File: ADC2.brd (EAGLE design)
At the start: 90 x 99 mm, 192 parts, among them CON1 USB-A, CON2 SWD_CON, IC1 STM32G431, IC10 NJM11100, IC11 TAR5SB33, IC12 LM4562, IC13 LM4562, IC14 NJM12888F18, IC15 AZ1117-3.3, IC16 -9V, IC17 +9V, IC18 LM4562, IC19 TC7WH74FU, IC2 7404, IC20 NJM2845-33, IC21 -5V, IC3 ESP32-WROVER, IC4 LME49721, IC5 TL431, IC6 AD4001, IC7 OCT_BUFFER-SO6, IC8 OCT_BUFFER-SO6, IC9 TAR5SB33, J2 SJ-1608, J4 SJ-1608, J5 SJ-2012, J6 IN1_DC, J7 SJ-1608, J8 short, J9 SJ-2012, SW1 Gain, X1 12MHz

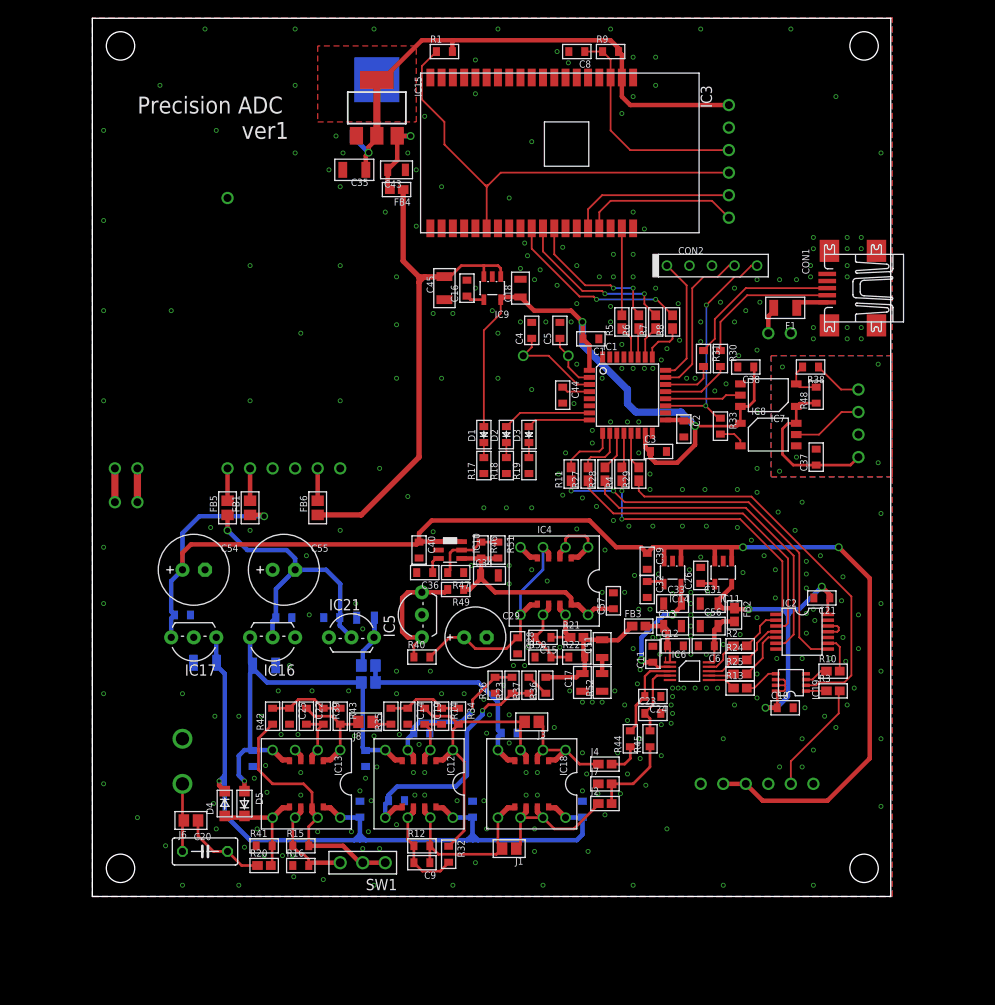
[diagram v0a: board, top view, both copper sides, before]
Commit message: ver2修正
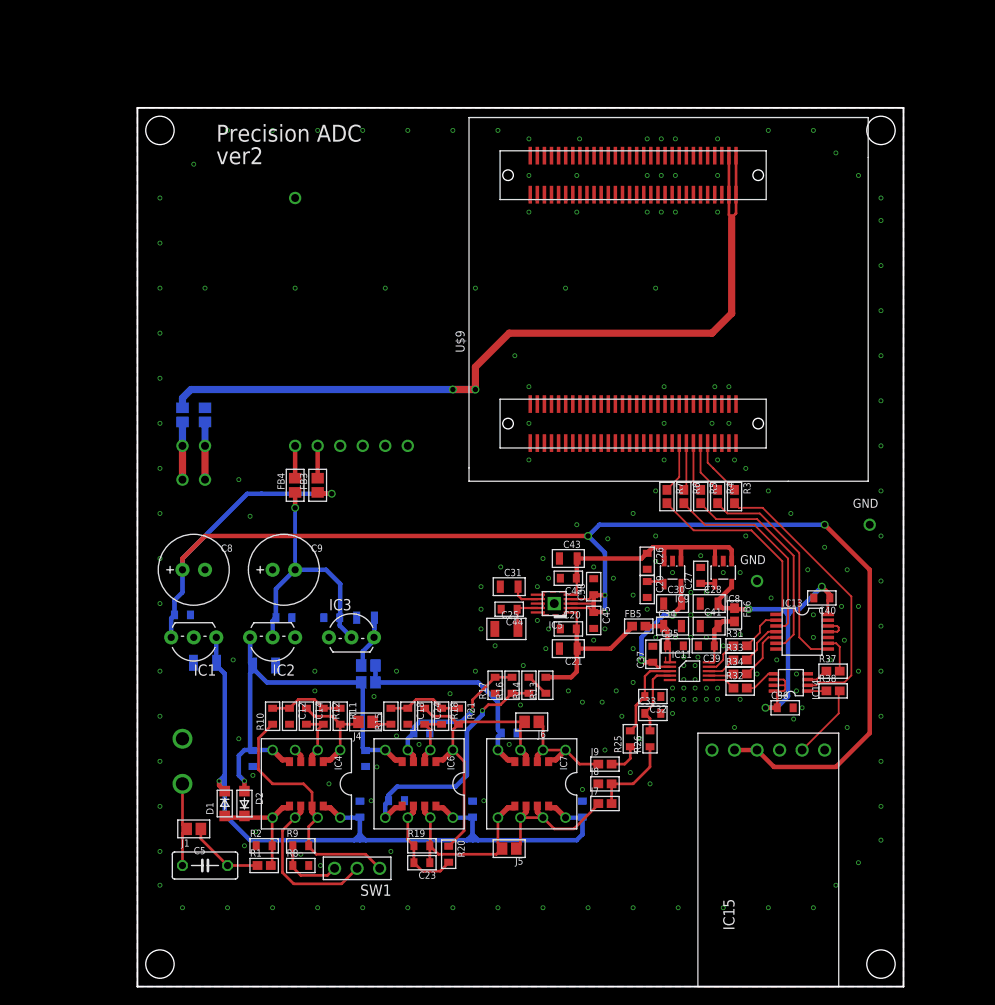
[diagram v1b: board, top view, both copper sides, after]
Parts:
- removed C46, C47: 10u, my_rcl:3216
- removed C48, C49, C50, C52, C53, C57, C59: 0.1u, my_rcl:1608
- removed C51, R52: DNP, my_rcl:2012
- removed C54, C55: 100u, my_rcl:E2,5-8
- removed C56, C58: 10u, my_rcl:2012
- removed CON1: USB-A, my_connector:UX60A-MB-5ST
- removed CON2: SWD_CON, my_connector:SWD_CON
- removed D3: ERR, my_rcl:D1608
- removed D4, D5: CLAMP, my_rcl:SOD123
- removed F1: 0.5A, my_rcl:3216
- removed IC10: NJM11100, my_ic:SOT23-6
- removed IC12, IC18: LM4562, my_ic:DIL8-SOP8
- removed IC16: -9V, my_ic:TO-92
- removed IC17: +9V, my_ic:TO-92
- removed IC19: TC7WH74FU, my_ic:SSOP8-P-0.65
- removed IC20: NJM2845-33, my_ic:P-HSIP3_2.30A
- removed IC21: -5V, my_ic:TO-92
- removed R22, R23, R35, R36, R39, R42, R43, R48, R49, R50: 1k, my_rcl:1608
- removed R24, R27, R28, R29: 37, my_rcl:1608-J
- removed R30, R44, R45: 22, my_rcl:1608
- removed R40, R46, R51: 10k, my_rcl:1608
- removed R41: 100k, my_rcl:1608
- removed R47: 1.5k, my_rcl:1608
- removed TP10: ESP_EN, my_connector:TESTPIN
- removed TP11: ESP_BOOT, my_connector:TESTPIN
- removed TP12: ESP_TX, my_connector:TESTPIN
- removed TP13, TP20, TP27, TP28, TP29: GND, my_connector:TESTPIN
- removed TP14: ESP_RX, my_connector:TESTPIN
- removed TP24: VDD_OSC, my_connector:TESTPIN
- removed TP25: OSC_EN, my_connector:TESTPIN
- removed TP26: OSC_OUT, my_connector:TESTPIN
- removed TP6: UART_RX, my_connector:TESTPIN
- removed TP7: UART_GND, my_connector:TESTPIN
- removed TP8: UART_TX, my_connector:TESTPIN
- removed TP9: +3V3D, my_connector:TESTPIN
- removed X1: 12MHz, my_rcl:HC49/S
- added U$9: FPGA_CORE_BOARD, my_ic:FPGA_CORE_BOARD
- C12: value 3300p -> 470p
- C13: value 10u -> 0.1u; device my_rcl:2012 -> my_rcl:1608
- C14, C24: value 470p -> 100p
- C15: value DNP -> 10u; device my_rcl:1608 -> my_rcl:2012
- C16: value 0.1u -> 10u; device my_rcl:1608 -> my_rcl:3216
- C17: device my_rcl:2012 -> my_rcl:3216
- C18, C33: value 10u -> 470p; device my_rcl:2012 -> my_rcl:1608
- C19, C22: value 100p -> 0.1u
- C20: value 10u -> 1u; device my_rcl:C050 -> my_rcl:1608
- C21, C30, C41: value 0.1u -> 10u; device my_rcl:1608 -> my_rcl:2012
- C23: value 470p -> DNP
- C25: value 470p -> 10u; device my_rcl:1608 -> my_rcl:3216
- C28: value 1u -> 10u; device my_rcl:1608 -> my_rcl:2012
- C29: value 100u -> 0.1u; device my_rcl:E2.5-6.5 -> my_rcl:1608
- C3: value 0.01u -> 0.1u
- C32: value 0.1u -> 470p
- C35: value 10u -> 3300p; device my_rcl:3216 -> my_rcl:1608
- C38, C42: value 0.1u -> 1u
- C4: value 22p -> 0.1u
- C44: value 0.1u -> DNP
- C45: value 10u -> 1u; device my_rcl:3216 -> my_rcl:1608
- C5: value 22p -> 10u; device my_rcl:1608 -> my_rcl:C050
- C8: value 0.1u -> 100u; device my_rcl:1608 -> my_rcl:E2,5-8
- C9: value DNP -> 100u; device my_rcl:1608 -> my_rcl:E2,5-8
- D1: value PWR -> CLAMP; device my_rcl:D1608 -> my_rcl:SOD123
- D2: value OK -> CLAMP; device my_rcl:D1608 -> my_rcl:SOD123
- FB2, FB3, FB4: value FB -> FB-2012; device my_rcl:1608-J -> my_rcl:2012-J
- FB5, FB6: value FB-2012 -> FB; device my_rcl:2012-J -> my_rcl:1608-J
- IC1: value STM32G431 -> +9V; device my_ic:TQFP32-08 -> my_ic:TO-92
- IC11: value TAR5SB33 -> AD4001; device my_ic:SOT23-5 -> my_ic:MSOP10
- IC13: value LM4562 -> 7404; device my_ic:DIL8-SOP8 -> my_ic:TSSOP14
- IC14: value NJM12888F18 -> TC7WH74FU; device my_ic:SOT23-5 -> my_ic:SSOP8-P-0.65
- IC15: value AZ1117-3.3 -> OSC; device my_ic:SOT223 -> my_ic:MY_OSC
- IC2: value 7404 -> -9V; device my_ic:TSSOP14 -> my_ic:TO-92
- IC3: value ESP32-WROVER -> -5V; device my_ic:ESP32-WROVER -> my_ic:TO-92
- IC4: value LME49721 -> LM4562
- IC5: value TL431 -> AK1110; device my_ic:TO-92 -> my_ic:PLP10
- IC6: value AD4001 -> LM4562; device my_ic:MSOP10 -> my_ic:DIL8-SOP8
- IC7: value OCT_BUFFER-SO6 -> LM4562; device my_ic:SO6 -> my_ic:DIL8-SOP8
- IC8: value OCT_BUFFER-SO6 -> TAR5SB33; device my_ic:SO6 -> my_ic:SOT23-5
- IC9: value TAR5SB33 -> NJM12888F18
- J1: value (none) -> IN1_DC
- J2: value SJ-1608 -> SJ-2012; device my_rcl:1608-J -> my_rcl:2012-J
- J3: value (none) -> SJ-2012
- J4: value SJ-1608 -> short; device my_rcl:1608-J -> my_rcl:2012-J
- J6: value IN1_DC -> SJ-2012
- J8: value short -> SJ-1608; device my_rcl:2012-J -> my_rcl:1608-J
- J9: value SJ-2012 -> SJ-1608; device my_rcl:2012-J -> my_rcl:1608-J
- R1: value 10k -> 10; device my_rcl:1608 -> my_rcl:1608-J
- R10, R11, R13, R8: value 37 -> 1k; device my_rcl:1608-J -> my_rcl:1608
- R15: value 10k -> 1k
- R17, R18, R19: value 1.5k -> 1k
- R2: value 37 -> 100k; device my_rcl:1608-J -> my_rcl:1608
- R20: value 10 -> 1k; device my_rcl:1608-J -> my_rcl:1608
- R21: value short -> 1k; device my_rcl:1608-J -> my_rcl:1608
- R25: value 37 -> 22; device my_rcl:1608-J -> my_rcl:1608
- R26: value 1k -> 22
- R3, R4, R5, R6, R7: value 37 -> 22
- R31: value 22 -> 37; device my_rcl:1608 -> my_rcl:1608-J
- R32, R33, R34, R37, R38: value 1k -> 37; device my_rcl:1608 -> my_rcl:1608-J
- TP4: value VBUS -> GND
- TP5: value UART_3V3 -> GND
- moved R9 96.1 mm to (23.5, 5.71)
- moved R1 94.0 mm to (19.4, 3.49)
- moved IC15 84.8 mm to (76.2, 16.5), turned to 90 degrees
- moved R8 74.2 mm to (23.5, 3.49), turned to 0 degrees
- moved C8 72.6 mm to (11.4, 36.8), turned to 0 degrees
- moved C5 72.4 mm to (12.7, 3.49), turned to 0 degrees
- moved C10 68.7 mm to (10.2, 31.8), flipped to the bottom, turned to 180 degrees
- moved C35 64.7 mm to (65.7, 28.3), turned to 0 degrees
- moved FB2 63.8 mm to (12.7, 54.3), flipped to the bottom
- moved R10 63.4 mm to (20.3, 20.3), turned to 90 degrees
- moved C2 61.2 mm to (18.1, 15.6), flipped to the bottom, turned to 90 degrees
- moved IC2 59.7 mm to (20.3, 29.2), turned to 180 degrees
- moved C1 59.1 mm to (30.2, 9.84), flipped to the bottom, turned to 90 degrees
- moved IC13 58.5 mm to (80.0, 29.8), turned to 270 degrees
- moved IC3 58.3 mm to (29.2, 29.2), turned to 0 degrees
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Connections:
- removed net +3V3: C1.2, C18.1, C2.1, C3.1, C38.1, D1.A, IC1.1, IC1.15, IC1.17, IC7.6, IC8.1, IC9.5
- removed net +3V3D: C35.1, IC15.2, IC15.4, IC20.3, IC3.2, R1.2, R9.2, TP9.1
- removed net +5.3V: C34.1, C57.1, IC10.4, IC4.1-8, IC4.2-8, R46.2, R49.1, R51.2
- removed net +5VD: C45.1, FB4.1, FB6.2, IC9.1, IC9.3
- removed net ADC1+: J4.2, R44.1
- removed net ADC1-: J2.2, J7.2, R45.1
- removed net ESP_BOOT: IC3.25, R1.1, TP11.1
- removed net ESP_EN: C8.1, IC3.3, R9.1, TP10.1
- removed net ESP_RX: IC3.34, TP14.1
- removed net ESP_TX: IC3.35, TP12.1
- removed net N$23: C15.1, IC4.1-7, IC4.2-7, R21.1
- removed net N$27: D1.K, R17.2
- removed net N$32: CON1.2, R30.1
- removed net N$33: CON1.3, R31.1
- removed net N$34: IC8.3, R33.2
- removed net N$35: IC7.3, R38.2, R48.2
- removed net N$36: IC1.10, R27.2
- removed net N$37: IC1.11, R28.2
- removed net N$39: IC13.1-6, IC13.2-6, R15.1, R16.2, SW1.3
- removed net N$40: D2.K, R18.2
- removed net N$46: D3.K, R19.2
- removed net N$50: D3.A, IC1.8
- removed net N$51: C16.1, IC9.4
- removed net N$52: C24.2, IC6.3, R44.2
- removed net N$53: C23.1, IC6.4, R45.2
- removed net N$54: D2.A, IC1.7
- removed net N$58: C15.2, IC4.1-6, IC4.2-6, R22.1, R50.2
- removed net N$60: IC5.1, IC5.3, R40.1, R49.2
- removed net N$61: C36.1, IC10.3
- removed net N$62: IC10.5, R46.1, R47.2, R51.1
- removed net N$63: C28.1, C29.+, IC4.1-3, IC4.1-5, IC4.2-3, IC4.2-5, R40.2
- removed net N$64: IC4.1-1, IC4.1-2, IC4.2-1, IC4.2-2
- removed net N$65: F1.2, TP4.1
- removed net N$66: C44.1, IC1.4
- removed net N$69: C43.1, FB4.2, IC15.3, IC20.1
- removed net N$72: FB6.1, TP1.1
- removed net N$73: C51.2, R52.2
- removed net SPI_CS: IC3.29, R8.2
- removed net SPI_MISO: IC3.31, R6.2
- removed net SPI_MOSI: IC3.37, R5.2
- removed net SPI_SCK: IC3.30, R7.2
- removed net STM_RX: IC1.20, IC7.5
- removed net STM_TX: CON2.5, IC1.19, R33.1
- removed net SWCLK: CON2.1, IC1.24
- removed net SWDIO: CON2.4, IC1.23
- removed net UART_3V3: C37.1, IC7.1, IC8.6, R48.1, TP5.1
- removed net UART_GND: C37.2, IC8.4, TP7.1
- removed net UART_RX: R38.1, TP6.1
- removed net UART_TX: IC8.5, TP8.1
- removed net USB_DM: IC1.21, R30.2
- removed net USB_DP: IC1.22, R31.2
- removed net VBUS: CON1.1, F1.1
- new net +5V: C26.1, C42.1, C43.1, IC5.5, IC8.1, IC8.3, IC9.1, IC9.3
- new net ADC+: J9.2, R25.1
- new net ADC+_LPF: C32.2, IC11.3, R25.2
- new net ADC-: J7.2, J8.2, R26.1
- new net ADC-_LPF: C33.1, IC11.4, R26.2
- new net VIN: FB1.1, U$9.117, U$9.118, U$9.119, U$9.120
- net +1V8: now also C30.1, C37.1, IC11.2, IC9.5; no longer C11.1, C33.1, IC14.5, IC6.2
- net +3V3A: now also C28.1, C36.1, C40.1, FB6.1, IC13.14, IC14.6, IC14.7, IC14.8, IC8.5; no longer C10.1, C21.1, C31.1, FB2.1, IC11.5, IC19.6, IC19.7, IC19.8, IC2.14
- net +9V: now also C1.1, C16.1, C3.1, C6.1, D1.2, IC1.1, IC4.1-8, IC4.2-8, IC6.1-8, IC6.2-8, IC7.1-8, IC7.2-8; no longer C41.1, C46.1, C48.1, C7.1, D4.2, IC12.1-8, IC12.2-8, IC13.1-8, IC13.2-8, IC17.1, IC18.1-8, IC18.2-8
- net -5V: now also C15.2, IC3.3, J3.1; no longer C58.2, IC21.3, J9.1
- net -9V: now also C17.2, C2.2, C4.2, D2.1, IC2.3, IC4.1-4, IC4.2-4, IC6.1-4, IC6.2-4, J2.1; no longer C42.2, C47.2, C49.2, D5.1, IC12.1-4, IC12.2-4, IC13.1-4, IC13.2-4, IC16.3, J5.1
- net ADC_CNVST: now also IC14.2, R3.2; no longer IC19.2, R29.1
- net ADC_CNVST_CLOCKED: now also IC14.5, R32.2; no longer IC19.5, R13.2
- net ADC_CNVST_FB: now also IC13.8, R4.2; no longer IC2.8, R11.1
- net ADC_SCK: now also IC13.3, R6.2; no longer IC2.3, R27.1
- net ADC_SDI: now also IC13.1, R7.2; no longer IC2.1, R4.1
- net ADC_SDO: now also IC13.6, R5.2; no longer IC2.6, R28.1
- net CLK_8MHZ: now also IC15.5, R38.2; no longer R3.2, TP26.1
- net GND: now also C1.2, C11.1, C13.1, C15.1, C17.1, C19.2, C2.1, C20.2, C22.2, C29.2, C32.1, C37.2, C4.1, C42.2, C7.1, C8.-, C9.+, FB2.1, IC1.2, IC11.5, IC13.13, IC13.7, IC14.4, IC15.4, IC15.6, IC2.1, IC4.1-3, IC4.2-3, IC5.10, IC5.6, IC5.8, IC5.HT, IC8.2, J8.1, R2.1, R8.2, TP4.1, TP5.1, U$9.1, U$9.101, U$9.102, U$9.103, U$9.104, U$9.113, U$9.114, U$9.115, U$9.116, U$9.2, U$9.39, U$9.40, U$9.53, U$9.54, U$9.57, U$9.58, U$9.61, U$9.62, U$9.83, U$9.84; no longer C1.1, C11.2, C13.2, C14.2, C17.2, C2.2, C23.2, C24.1, C29.-, C32.2, C4.2, C42.1, C46.2, C47.1, C48.2, C49.1, C5.2, C50.1, C52.2, C53.1, C54.-, C55.+, C56.2, C57.2, C58.1, C59.1, C7.2, C8.2, CON1.5, CON1.M1, CON1.M2, CON1.M3, CON1.M4, CON2.3, IC1.14, IC1.16, IC1.31, IC1.32, IC10.2, IC11.2, IC13.1-3, IC13.2-3, IC14.2, IC16.1, IC17.2, IC19.4, IC2.13, IC2.7, IC20.2, IC21.1, IC3.15, IC3.38, IC4.1-4, IC4.2-4, IC5.2, IC6.5, IC7.4, J7.1, R16.1, R18.1, R19.1, R26.1, R41.1, R47.1, R50.1, R52.1, TP13.1, TP20.1, TP27.1, TP28.1, TP29.1
- net N$1: now also R8.1, R9.1, SW1.3; no longer C5.1, IC1.2, X1.2
- net N$10: now also R6.1, U$9.46; no longer IC1.12, R4.2
- net N$11: now also IC14.3, R37.1; no longer IC19.3, R10.1
- net N$12: now also C5.2, J1.2, R1.1; no longer C20.2, J6.2, R20.1
- net N$13: now also IC13.2, R31.2; no longer IC2.2, R2.2
- net N$14: now also C23.1, IC6.1-7, IC6.2-7, IC7.1-5, IC7.2-5, J5.2, R19.2; no longer C9.1, IC12.1-7, IC12.2-7, IC18.1-5, IC18.2-5, J1.2, R12.2
- net N$15: now also C39.1, C41.1, FB6.2, IC11.10; no longer C56.1, C6.1, FB2.2, IC6.10
- net N$16: now also C34.1, C35.1, FB5.2, IC11.1; no longer C12.1, C13.1, FB3.2, IC6.1
- net N$17: now also R5.1, U$9.48; no longer IC1.25, R8.1
- net N$18: now also IC14.1, R38.1; no longer IC19.1, R3.1
- net N$19: now also IC13.9, R37.2; no longer IC2.9, R10.2
- net N$2: now also IC7.1-6, IC7.1-7, IC7.2-6, IC7.2-7, J5.1, J7.1; no longer IC18.1-6, IC18.1-7, IC18.2-6, IC18.2-7, J1.1, J2.1
- net N$20: now also IC13.5, R34.2; no longer IC2.5, R25.2
- net N$21: now also R3.1, U$9.52; no longer IC1.9, R11.2
- net N$22: now also IC13.11, IC13.12; no longer IC2.11, IC2.12
- net N$24: now also J4.2, R15.1; no longer J8.2, R35.1
- net N$25: now also IC11.7, R34.1; no longer IC6.7, R25.1
- net N$26: now also C24.2, IC6.1-2, IC6.2-2, R18.2; no longer C19.2, IC12.1-2, IC12.2-2, R14.2
- net N$28: now also IC11.8, R33.1; no longer IC6.8, R24.1
- net N$29: now also IC11.6, R32.1; no longer IC6.6, R13.1
- net N$3: now also IC4.1-6, IC4.2-6, SW1.2; no longer C4.1, IC1.3, X1.1
- net N$30: now also IC11.9, R31.1; no longer IC6.9, R2.1
- net N$31: now also IC13.4, R33.2; no longer IC2.4, R24.2
- net N$38: now also R13.1, R14.2; no longer R36.1, R37.2
- net N$4: now also C12.1, R10.2, R11.1, R12.1; no longer C25.1, R39.1, R42.2, R43.1
- net N$41: now also C22.1, IC6.1-5, IC6.2-5, R14.1, R16.1; no longer C27.1, IC12.1-5, IC12.2-5, R23.1, R37.1
- net N$42: now also C23.2, IC6.1-6, IC6.2-6, R19.1, R20.2; no longer C9.2, IC12.1-6, IC12.2-6, R12.1, R32.2
- net N$43: now also C18.1, R15.2, R18.1, R21.1; no longer C14.1, R14.1, R34.1, R35.2
- net N$44: now also C19.1, IC6.1-3, IC6.2-3, R16.2, R17.2; no longer C30.1, IC12.1-3, IC12.2-3, R23.2, R26.2
- net N$45: now also IC4.1-7, IC4.2-7, R10.1, R9.2; no longer IC13.1-7, IC13.2-7, R15.2, R42.1, SW1.2
- net N$47: now also C24.1, IC6.1-1, IC6.2-1, IC7.1-3, IC7.2-3, J6.2, R20.1, R21.2; no longer C19.1, IC12.1-1, IC12.2-1, IC18.1-3, IC18.2-3, J3.2, R32.1, R34.2
- net N$48: now also C5.1, J1.1; no longer C20.1, J6.1
- net N$49: now also D1.1, D2.2, IC4.1-5, IC4.2-5, R1.2, R2.2; no longer D4.1, D5.2, IC13.1-5, IC13.2-5, R20.2, R41.2
- net N$5: now also IC7.1-1, IC7.1-2, IC7.2-1, IC7.2-2, J6.1, J9.1; no longer IC18.1-1, IC18.1-2, IC18.2-1, IC18.2-2, J3.1, J4.1
- net N$55: now also C14.2, IC4.1-2, IC4.2-2, R12.2; no longer C22.2, IC13.1-2, IC13.2-2, R39.2
- net N$56: now also C27.1, IC8.4; no longer C26.1, IC11.4
- net N$57: now also C14.1, IC4.1-1, IC4.2-1, J4.1, R11.2; no longer C22.1, IC13.1-1, IC13.2-1, J8.1, R43.2
- net N$59: now also C29.1, IC9.4; no longer C32.1, IC14.4
- net N$6: now also R4.1, U$9.50; no longer IC1.26, R7.1
- net N$7: now also C31.1, IC5.7; no longer IC1.27, R6.1
- net N$70: now also FB3.1; no longer FB1.1
- net N$71: now also FB4.1; no longer FB5.1
- net N$74: now also C7.2, IC7.1-4, IC7.2-4, J2.2, J3.2; no longer C50.2, IC18.1-4, IC18.2-4, J5.2, J9.2
- net N$75: now also FB1.2
- net N$76: now also FB2.2
- net N$8: now also C25.1, C44.1, IC5.9; no longer IC1.28, R5.1
- net N$9: now also R7.1, U$9.44; no longer IC1.13, R29.2
- net V+: now also C10.1, C38.1, C45.1, C8.+, FB3.2, IC1.3, IC15.2, IC15.3, IC5.2, IC5.3, IC5.4; no longer C39.1, C40.1, C52.1, C54.+, FB1.2, IC10.1, IC10.6, IC11.1, IC11.3, IC14.1, IC14.3, IC17.3, TP24.1, TP25.1
- net V-: now also C11.2, C13.2, C9.-, FB4.2, IC2.2, IC3.2; no longer C53.2, C55.-, C59.2, FB5.2, IC16.2, IC21.2
- net VREF: now also C20.1, C21.1, FB5.1, IC5.1, R13.2; no longer C17.1, C51.1, FB3.1, R21.2, R22.2, R36.2
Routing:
- net VIN: track 0.00 -> 96.1 mm, vias 0 -> 2
- net +3V3: track 79.1 -> 0.00 mm, vias 2 -> 0
- net +3V3D: track 62.0 -> 0.00 mm, vias 1 -> 0
- net +5VD: track 58.3 -> 0.00 mm
- net ESP_BOOT: track 51.9 -> 0.00 mm
- net +5V: track 0.00 -> 31.0 mm
- net N$63: track 27.1 -> 0.00 mm
- net +5.3V: track 26.6 -> 0.00 mm
- net STM_TX: track 25.7 -> 0.00 mm, vias 2 -> 0
- net ESP_EN: track 25.5 -> 0.00 mm
- net SPI_CS: track 21.3 -> 0.00 mm, vias 2 -> 0
- net SPI_SCK: track 19.0 -> 0.00 mm, vias 2 -> 0
- net ESP_RX: track 18.7 -> 0.00 mm
- net UART_3V3: track 18.4 -> 0.00 mm
- net ADC_CNVST_FB: track 43.1 -> 24.8 mm, vias 2 -> 0
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- removed copper zone on layer 1, net +3V3D
- removed copper zone on layer 15, net N$67
- removed copper zone on layer 2, net N$68
- removed copper zone on layer 1, net UART_GND
- removed copper zone on layer 16, net UART_GND
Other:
- board size 90 x 99 mm -> 86.4 x 99.1 mm
- board text added: "ver2"
- board text removed: "ver1"

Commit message: update
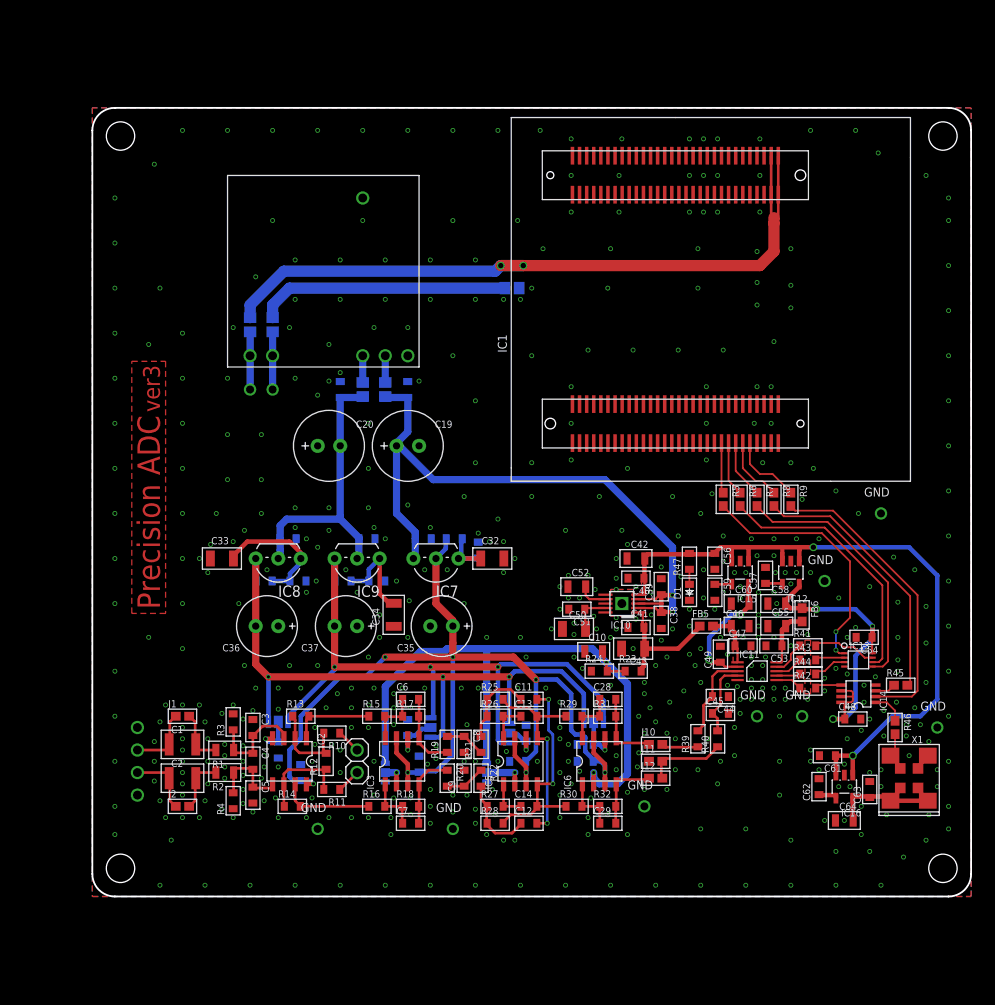
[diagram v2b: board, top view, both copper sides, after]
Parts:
- removed D2: CLAMP, my_rcl:SOD123
- removed SW1: Gain, my_connector:1X03
- removed TP15: -D5V, my_connector:TESTPIN
- removed TP16: GND, my_connector:TESTPIN-BIG
- removed TP17: V+, my_connector:TESTPIN
- removed TP18: GND, my_connector:TESTPIN
- removed TP19: V-, my_connector:TESTPIN
- removed TP21: VIN+, my_connector:TESTPIN
- removed TP22: VIN-, my_connector:TESTPIN
- removed TP23: (no value), my_connector:TESTPIN
- removed U$9: FPGA_CORE_BOARD, my_ic:FPGA_CORE_BOARD
- added C46, C52, C55, C58, C60, C64: 10u, my_rcl:2012
- added C47: 3300p, my_rcl:1608C
- added C48, C49, C53, C54, C56, C57, C59, C61, C62, C63: 0.1u, my_rcl:1608C
- added C50: 10u, my_rcl:3216
- added C51: DNP, my_rcl:1608C
- added IC10: AK1110, my_ic:PLP10
- added IC12, IC16: TAR5SB33, my_ic:SOT23-5
- added J10: ADC+, my_rcl:1608-J
- added J11: GND, my_rcl:1608-J
- added J12: ADC-, my_rcl:1608-J
- added JP1: GAIN, my_connector:1X02
- added R22, R23, R24, R27, R29, R30: 1k, my_rcl:1608
- added R28: 3.6k, my_rcl:1608
- added R35: 330, my_rcl:1608
- added R36: 120, my_rcl:1608
- added R39, R40: 22, my_rcl:1608
- added R41, R42, R43, R44: 37, my_rcl:1608
- added R45, R46: 37, my_rcl:1608-J
- added R47: 5.1k, my_rcl:1608
- added TP10, TP11, TP12, TP7, TP8, TP9: GND, my_connector:TESTPIN
- added TP6: AIN-, my_connector:TESTPIN-MID
- added X1: 12MHz, my_rcl:KC7050
- C1, C2: value 0.1u -> 1u; device my_rcl:1608 -> my_rcl:3225
- C10: value 0.1u -> 10u; device my_rcl:1608 -> my_rcl:2012
- C11: value 0.1u -> 1n; device my_rcl:1608 -> my_rcl:1608C
- C12: value 470p -> 1n; device my_rcl:1608 -> my_rcl:1608C
- C13: value 0.1u -> 1.5n; device my_rcl:1608 -> my_rcl:1608C
- C14: value 100p -> 1.5n; device my_rcl:1608 -> my_rcl:1608C
- C15, C41: value 10u -> 1u; device my_rcl:2012 -> my_rcl:1608C
- C16: value 10u -> 1u; device my_rcl:3216 -> my_rcl:1608C
- C17, C25: value 10u -> 0.1u; device my_rcl:3216 -> my_rcl:1608C
- C18: value 470p -> 0.1u; device my_rcl:1608 -> my_rcl:1608C
- C19: value 0.1u -> 100u; device my_rcl:1608 -> my_rcl:E2,5-8
- C20: value 1u -> 100u; device my_rcl:1608 -> my_rcl:E2,5-8
- C21, C30, C31: value 10u -> 0.1u; device my_rcl:2012 -> my_rcl:1608C
- C22, C26, C27, C38: device my_rcl:1608 -> my_rcl:1608C
- C23: value DNP -> 0.1u; device my_rcl:1608 -> my_rcl:1608C
- C24: value 100p -> 0.1u; device my_rcl:1608 -> my_rcl:1608C
- C28: value 10u -> 10p; device my_rcl:2012 -> my_rcl:1608C
- C29, C6, C7: value 0.1u -> 10p; device my_rcl:1608 -> my_rcl:1608C
- C3, C4: value 0.1u -> DNP; device my_rcl:1608 -> my_rcl:1608C
- C32, C33: value 470p -> 10u; device my_rcl:1608 -> my_rcl:3216
- C34, C43: device my_rcl:2012 -> my_rcl:3216
- C35: value 3300p -> 100u; device my_rcl:1608 -> my_rcl:E2.5-6.5
- C36, C37: value 0.1u -> 100u; device my_rcl:1608 -> my_rcl:E2.5-6.5
- C39, C40: value 0.1u -> 1u; device my_rcl:1608 -> my_rcl:1608C
- C42: value 1u -> 10u; device my_rcl:1608 -> my_rcl:2012
- C44: value DNP -> 470p; device my_rcl:1608 -> my_rcl:1608C
- C45: value 1u -> 470p; device my_rcl:1608 -> my_rcl:1608C
- C5: value 10u -> DNP; device my_rcl:C050 -> my_rcl:1608C
- C8, C9: value 100u -> 2.7n; device my_rcl:E2,5-8 -> my_rcl:1608C
- D1: value CLAMP -> PWR; device my_rcl:SOD123 -> my_rcl:D1608
- FB1, FB2, FB3, FB4: value FB-2012 -> FB
- IC1: value +9V -> FPGA CORE BOARD; device my_ic:TO-92 -> my_ic:FPGA_CORE_BOARD
- IC13: value 7404 -> 74HC3G34; device my_ic:TSSOP14 -> my_ic:SOT765
- IC15: value OSC -> NJM12888F18; device my_ic:MY_OSC -> my_ic:SOT23-5
- IC2: value -9V -> OPA; device my_ic:TO-92 -> my_ic:SOP8
- IC3: value -5V -> OPA-DIFF; device my_ic:TO-92 -> my_ic:SOP8
- IC4: value LM4562 -> DCDC2; device my_ic:DIL8-SOP8 -> my_ic:DCDC2
- IC5: value AK1110 -> OPA-DIFF; device my_ic:PLP10 -> my_ic:SOP8
- IC6: value LM4562 -> OPA-DIFF; device my_ic:DIL8-SOP8 -> my_ic:SOP8
- IC7: value LM4562 -> LM317-L; device my_ic:DIL8-SOP8 -> my_ic:TO-92
- IC8: value TAR5SB33 -> LM337-L; device my_ic:SOT23-5 -> my_ic:TO-92
- IC9: value NJM12888F18 -> LM337-L; device my_ic:SOT23-5 -> my_ic:TO-92
- J1: value IN1_DC -> DC; device my_rcl:2012-J -> my_rcl:1608-J
- J2: value SJ-2012 -> DC; device my_rcl:2012-J -> my_rcl:1608-J
- J3, J5: value SJ-2012 -> VCOM; device my_rcl:2012-J -> my_rcl:1608-3-J
- J4: value short -> GND
- J6: value SJ-2012 -> V-; device my_rcl:2012-J -> my_rcl:2012-3-J
- J7, J8, J9: value SJ-1608 -> V-; device my_rcl:1608-J -> my_rcl:2012-3-J
- R1: device my_rcl:1608-J -> my_rcl:2012
- R10, R11: value 1k -> 100
- R2: value 100k -> 10; device my_rcl:1608 -> my_rcl:2012
- R25: value 22 -> 3.6k
- R26: value 22 -> 1k
- R3, R4: value 22 -> 10k; device my_rcl:1608-J -> my_rcl:1608
- R31, R32: value 37 -> 1k; device my_rcl:1608-J -> my_rcl:1608
- R33, R34: value 37 -> 680; device my_rcl:1608-J -> my_rcl:1608
- R37, R38: value 37 -> 120; device my_rcl:1608-J -> my_rcl:1608
- R8: value 1k -> 22; device my_rcl:1608 -> my_rcl:1608-J
- R9: value 10k -> 22; device my_rcl:1608 -> my_rcl:1608-J
- TP1: value +D5V -> GND; device my_connector:TESTPIN -> my_connector:TESTPIN-MID
- TP2: value AIN1 -> AIN+; device my_connector:TESTPIN-BIG -> my_connector:TESTPIN-MID
- TP3: device my_connector:TESTPIN -> my_connector:TESTPIN-MID
- moved R9 67.7 mm to (78.7, 44.8), turned to 270 degrees
- moved R8 67.4 mm to (76.8, 44.8), turned to 270 degrees
- moved IC1 66.3 mm to (65.7, 67.3), turned to 0 degrees
- moved R37 64.9 mm to (19.4, 35.6), flipped to the bottom
- moved R4 64.5 mm to (15.9, 10.8), turned to 90 degrees
- moved R3 62.0 mm to (15.9, 19.7), turned to 90 degrees
- moved C36 59.1 mm to (19.7, 30.5), turned to 180 degrees
- moved D1 57.5 mm to (67.3, 34.3)
- moved R38 56.6 mm to (28.3, 35.6), flipped to the bottom
- moved C33 51.6 mm to (14.6, 38.1)
- moved J4 51.6 mm to (47.3, 68.6), flipped to the bottom
- moved R34 50.9 mm to (23.2, 35.6), flipped to the bottom, turned to 180 degrees
- moved IC8 50.2 mm to (21.0, 38.1)
- moved IC4 48.7 mm to (30.5, 61.0), turned to 0 degrees
- moved TP1 48.3 mm to (5.08, 11.4)
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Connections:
- new net ADC_VCOM: C10.1, IC6.2, J3.3, J5.3, R23.1, R24.2
- new net N$23: C4.2, C5.1, IC2.5, R2.2, R4.2
- new net N$27: C13.1, IC5.8, R26.2
- new net N$32: C12.2, C13.2, IC5.5, R25.2, R29.1
- new net N$33: C11.2, C14.2, IC5.4, R28.2, R30.1
- new net N$34: C14.1, IC5.1, R27.2
- new net N$35: C12.1, R22.2, R27.1, R28.1
- new net N$36: C11.1, R21.2, R25.1, R26.1
- new net N$37: C7.2, IC3.4, R18.2, R20.1
- new net N$39: C7.1, IC3.1, R16.2, R18.1
- new net N$40: C6.1, IC3.8, R15.2, R17.1
- new net N$46: JP1.2, R11.1
- new net N$50: C27.2, IC5.6, J8.2
- new net N$51: C22.2, IC3.6, J7.2
- new net N$52: C18.2, IC2.4, J6.2
- new net N$53: C32.1, IC7.1, R33.2, R36.1
- new net N$54: C33.2, IC8.1, R34.1, R37.1
- new net N$58: D1.A, R47.1
- new net VCC_OSC: C63.1, C64.1, IC16.5, X1.1, X1.1-2, X1.4, X1.4-2
- net +1V8: now also C49.1, C60.1, IC15.5; no longer C30.1, C37.1, IC9.5
- net +3V3A: now also C48.1, C54.1, C58.1, IC12.5, IC13.8; no longer C28.1, C36.1, C40.1, IC13.14, IC8.5
- net +5V: now also C40.1, C56.1, C61.1, IC10.5, IC12.1, IC12.3, IC15.1, IC15.3, IC16.1, IC16.3, R47.2; no longer C26.1, C43.1, IC5.5, IC8.1, IC8.3, IC9.1, IC9.3
- net +9V: now also C17.1, C21.1, C26.1, C30.1, C35.+, IC2.8, IC3.3, IC3.7, IC5.3, IC5.7, IC6.3, IC6.7, IC7.2, R36.2; no longer C1.1, C16.1, C3.1, C6.1, D1.2, IC1.1, IC4.1-8, IC4.2-8, IC6.1-8, IC6.2-8, IC7.1-8, IC7.2-8
- net -5V: now also C37.-, IC9.3, J6.1, J7.1, J8.1, J9.1, R38.2; no longer C15.2, IC3.3, J3.1
- net -9V: now also C36.-, IC8.3, J6.3, J7.3, J8.3, J9.3, R37.2; no longer C17.2, C2.2, C4.2, D2.1, IC2.3, IC4.1-4, IC4.2-4, IC6.1-4, IC6.2-4, J2.1
- net ADC+: now also J10.2, R39.1; no longer J9.2, R25.1
- net ADC+_LPF: now also C44.2, R39.2; no longer C32.2, R25.2
- net ADC-: now also J11.2, J12.2, R40.1; no longer J7.2, J8.2, R26.1
- net ADC-_LPF: now also C45.1, R40.2; no longer C33.1, R26.2
- net ADC_CNVST: now also R9.2; no longer R3.2
- net ADC_CNVST_CLOCKED: now also R42.2; no longer R32.2
- net ADC_CNVST_FB: now also R45.2, R8.2; no longer IC13.8, R4.2
- net ADC_SCK: now also IC13.6; no longer IC13.3
- net ADC_SDI: now also R5.2; no longer R7.2
- net ADC_SDO: now also IC13.5, R7.2; no longer IC13.6, R5.2
- net CLK_8MHZ: now also R46.2, X1.3, X1.3-2; no longer IC15.5, R38.2
- net GND: now also C15.2, C16.1, C17.2, C18.1, C19.-, C20.+, C22.1, C23.2, C24.1, C25.1, C27.1, C3.1, C31.1, C32.2, C33.1, C34.1, C35.-, C36.+, C37.+, C44.1, C46.2, C47.2, C48.2, C49.2, C5.2, C50.2, C51.2, C52.2, C53.2, C54.2, C55.2, C56.2, C57.2, C58.2, C59.2, C60.2, C61.2, C62.2, C63.2, C64.2, C8.2, C9.2, D1.K, IC1.1, IC1.101, IC1.102, IC1.103, IC1.104, IC1.113, IC1.114, IC1.115, IC1.116, IC1.39, IC1.40, IC1.53, IC1.54, IC1.57, IC1.58, IC1.61, IC1.62, IC1.83, IC1.84, IC10.10, IC10.6, IC10.8, IC10.HT, IC12.2, IC13.4, IC15.2, IC16.2, IC4.GND1, J11.1, J3.1, J4.1, J5.1, R24.1, R3.2, R33.1, R34.2, R35.2, R4.1, TP1.1, TP10.1, TP11.1, TP12.1, TP7.1, TP8.1, TP9.1, X1.2, X1.2-2; no longer C1.2, C11.1, C12.2, C13.1, C15.1, C16.2, C17.1, C18.2, C19.2, C2.1, C20.2, C22.2, C25.2, C27.2, C28.2, C29.2, C3.2, C31.2, C32.1, C33.2, C34.2, C35.2, C36.2, C37.2, C4.1, C44.2, C6.2, C7.1, C8.-, C9.+, FB2.1, IC13.13, IC13.7, IC15.1, IC15.4, IC15.6, IC2.1, IC3.1, IC4.1-3, IC4.2-3, IC5.10, IC5.6, IC5.8, IC5.HT, IC8.2, IC9.2, J8.1, R17.1, R2.1, R8.2, TP16.1, TP18.1, U$9.1, U$9.101, U$9.102, U$9.103, U$9.104, U$9.113, U$9.114, U$9.115, U$9.116, U$9.2, U$9.39, U$9.40, U$9.53, U$9.54, U$9.57, U$9.58, U$9.61, U$9.62, U$9.83, U$9.84
- net N$1: now also IC2.6, R11.2, R12.1, R14.1; no longer R8.1, R9.1, SW1.3
- net N$10: now also IC1.46; no longer U$9.46
- net N$11: now also R45.1; no longer R37.1
- net N$12: now also IC2.7, R14.2, R16.1; no longer C5.2, J1.2, R1.1
- net N$13: now also IC13.7, R41.2; no longer IC13.2, R31.2
- net N$14: now also C3.2, C4.1, IC2.3, R1.2, R3.1; no longer C23.1, IC6.1-7, IC6.2-7, IC7.1-5, IC7.2-5, J5.2, R19.2
- net N$15: now also C53.1, C55.1; no longer C39.1, C41.1
- net N$16: now also C46.1, C47.1; no longer C34.1, C35.1
- net N$17: now also IC1.48, R7.1; no longer R5.1, U$9.48
- net N$18: now also R46.1; no longer R38.1
- net N$19: now also C29.1, IC6.1, R30.2, R32.1; no longer IC13.9, R37.2
- net N$2: now also C29.2, IC6.4, J12.1, R32.2; no longer IC7.1-6, IC7.1-7, IC7.2-6, IC7.2-7, J5.1, J7.1
- net N$20: now also IC13.3, R44.2; no longer IC13.5, R34.2
- net N$21: now also IC1.52, R9.1; no longer R3.1, U$9.52
- net N$22: now also C28.1, IC6.8, R29.2, R31.1; no longer IC13.11, IC13.12
- net N$24: now also C8.1, R19.2, R21.1; no longer J4.2, R15.1
- net N$25: now also R44.1; no longer R34.1
- net N$26: now also C9.1, R20.2, R22.1; no longer C24.2, IC6.1-2, IC6.2-2, R18.2
- net N$28: now also R43.1; no longer R33.1
- net N$29: now also R42.1; no longer R32.1
- net N$3: now also IC2.2, R10.2, R12.2, R13.1; no longer IC4.1-6, IC4.2-6, SW1.2
- net N$30: now also R41.1; no longer R31.1
- net N$31: now also IC13.2, R43.2; no longer IC13.4, R33.2
- net N$38: now also C6.2, IC3.5, R17.2, R19.1; no longer R13.1, R14.2
- net N$4: now also IC2.1, R13.2, R15.1; no longer C12.1, R10.2, R11.1, R12.1
- net N$41: now also C1.1, J1.1, TP2.1; no longer C22.1, IC6.1-5, IC6.2-5, R14.1, R16.1
- net N$42: now also C2.1, J2.1, TP6.1; no longer C23.2, IC6.1-6, IC6.2-6, R19.1, R20.2
- net N$43: now also C1.2, J1.2, R1.1; no longer C18.1, R15.2, R18.1, R21.1
- net N$44: now also C2.2, J2.2, R2.1; no longer C19.1, IC6.1-3, IC6.2-3, R16.2, R17.2
- net N$45: now also JP1.1; no longer IC4.1-7, IC4.2-7, R9.2, SW1.1
- net N$47: now also IC5.2, J5.2; no longer C24.1, IC6.1-1, IC6.2-1, IC7.1-3, IC7.2-3, J6.2, R20.1, R21.2
- net N$48: now also C62.1, IC16.4; no longer C5.1, J1.1, TP2.1
- net N$49: now also IC3.2, J3.2; no longer D1.1, D2.2, IC4.1-5, IC4.2-5, R1.2, R2.2
- net N$5: now also C28.2, IC6.5, J10.1, R31.2; no longer IC7.1-1, IC7.1-2, IC7.2-1, IC7.2-2, J6.1, J9.1
- net N$55: now also C34.2, IC9.1, R35.1, R38.1; no longer C14.2, IC4.1-2, IC4.2-2, R12.2
- net N$56: now also C57.1, IC12.4; no longer C27.1, IC8.4
- net N$57: now also FB2.1, J4.2; no longer C14.1, IC4.1-1, IC4.2-1, J4.1, R11.2
- net N$59: now also C59.1, IC15.4; no longer C29.1, IC9.4
- net N$6: now also IC1.50, R8.1; no longer R4.1, U$9.50
- net N$7: now also C52.1, IC10.7; no longer C31.1, IC5.7
- net N$70: now also IC4.V+; no longer TP17.1
- net N$71: now also IC4.V-; no longer TP19.1
- net N$74: now also C31.2, IC6.6, J9.2; no longer C7.2, IC7.1-4, IC7.2-4, J2.2, J3.2
- net N$75: now also IC4.VIN+; no longer TP21.1
- net N$76: now also IC4.VIN-; no longer TP22.1
- net N$8: now also C50.1, C51.1, IC10.9; no longer C25.1, C44.1, IC5.9
- net N$9: now also IC1.44, R5.1; no longer R7.1, U$9.44
- net V+: now also C15.1, C19.+, C23.1, C39.1, IC10.2, IC10.3, IC10.4, IC7.3; no longer C10.1, C45.1, C8.+, IC1.3, IC15.2, IC15.3, IC5.2, IC5.3, IC5.4
- net V-: now also C16.2, C20.-, C24.2, C25.2, IC8.2, IC9.2; no longer C11.2, C13.2, C9.-, IC2.2, IC3.2
- net VIN: now also IC1.117, IC1.118, IC1.119, IC1.120; no longer U$9.117, U$9.118, U$9.119, U$9.120
- net VREF: now also C41.1, C43.1, IC10.1, R23.2; no longer C20.1, C21.1, IC5.1, R13.2
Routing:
- net V+: track 171.7 -> 78.2 mm, vias 5 -> 2
- net ADC_VCOM: track 0.00 -> 73.4 mm, vias 0 -> 2
- net -5V: track 6.01 -> 73.5 mm, vias 0 -> 3
- net +5V: track 31.0 -> 81.1 mm, vias 0 -> 2
- net N$47: track 34.8 -> 4.50 mm, vias 0 -> 1
- net +9V: track 90.5 -> 117.3 mm, vias 1 -> 7
- net N$45: track 28.7 -> 2.75 mm
- net -9V: track 49.4 -> 74.9 mm, vias 1 -> 3
- net N$33: track 0.00 -> 23.4 mm, vias 0 -> 2
- net N$32: track 0.00 -> 22.3 mm, vias 0 -> 2
- net N$41: track 29.0 -> 7.73 mm, vias 1 -> 0
- net N$74: track 25.7 -> 5.48 mm, vias 0 -> 1
- net VCC_OSC: track 0.00 -> 16.4 mm
- net N$57: track 12.1 -> 28.4 mm
- net N$54: track 0.00 -> 14.8 mm
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- added copper zone on layer 1, net +5V
- added copper zone on layer 1, net VREF
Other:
- board size 86.4 x 99.1 mm -> 99.1 x 88.9 mm
- board text added: "ver3"
- board text removed: "ver2"
